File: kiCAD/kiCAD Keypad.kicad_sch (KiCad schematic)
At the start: 71 parts, among them J1 USB_C_Receptacle_USB2.0_16P, J3 2x8 GPIO for SPI, SW1 RESET, SW2 BOOT, SW3 RotaryEncoder_Switch, U1 ESP32-S3-WROOM-2, U2 USBLC6-2SC6, U4 AP2112K-3.3

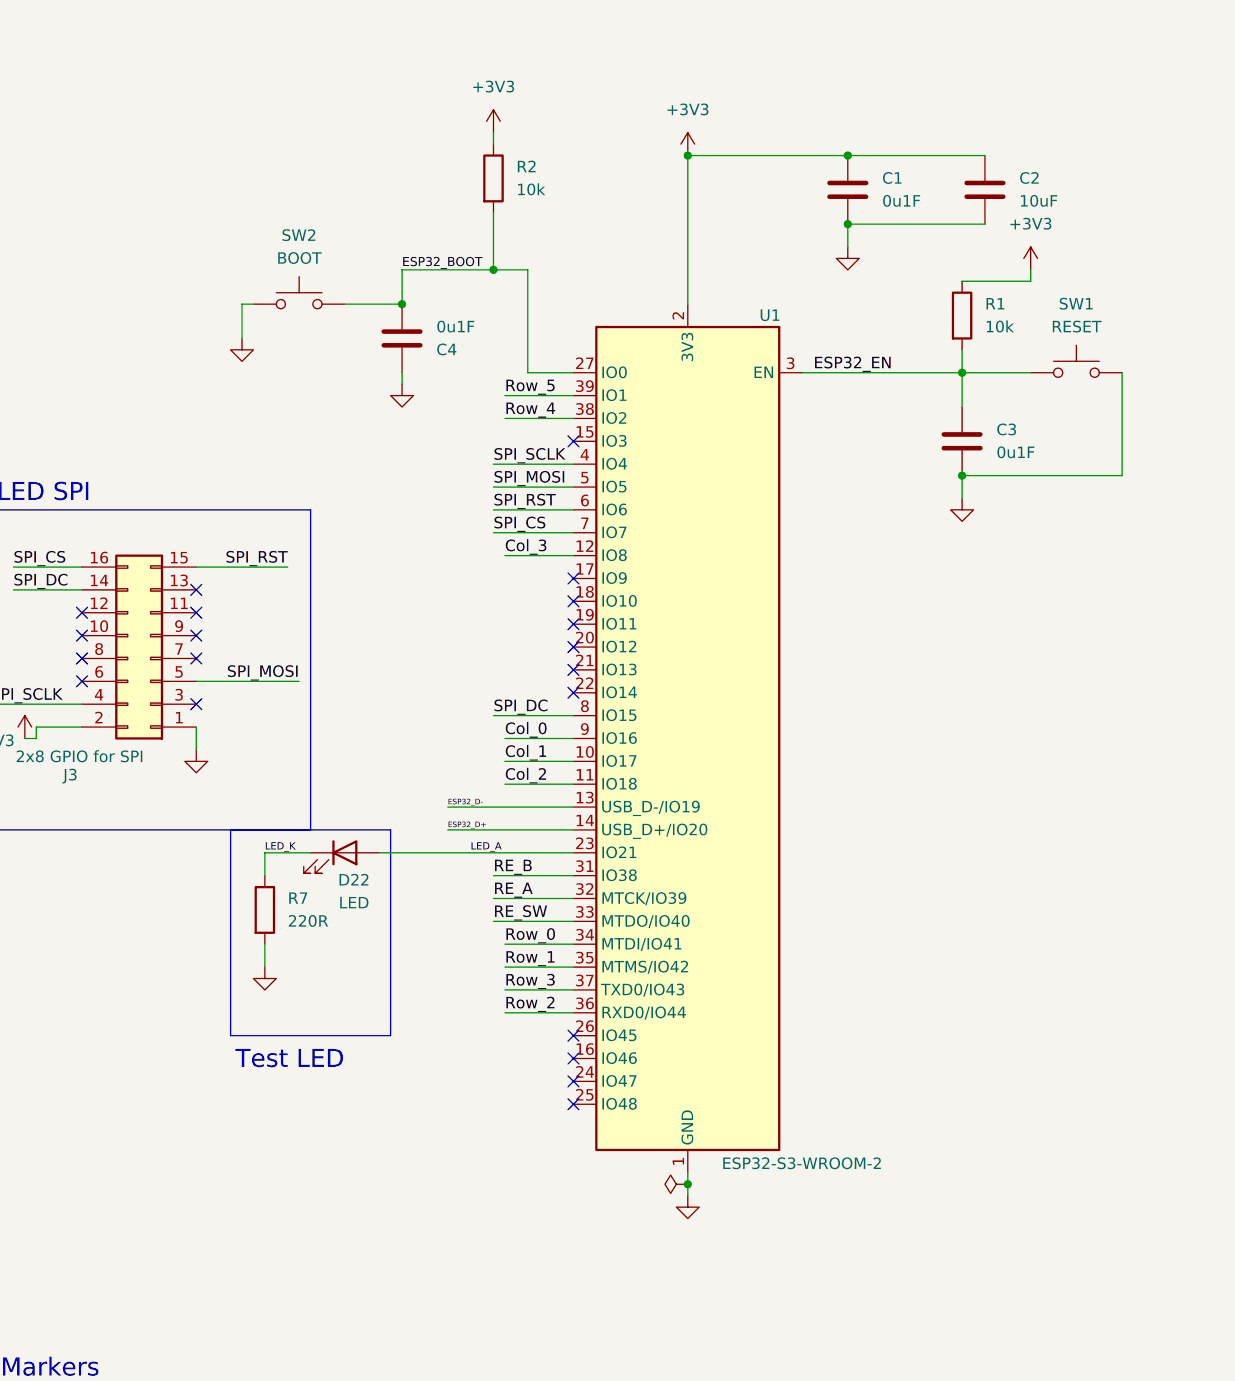
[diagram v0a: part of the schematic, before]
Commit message: Iterating; deciding on switching to devkit
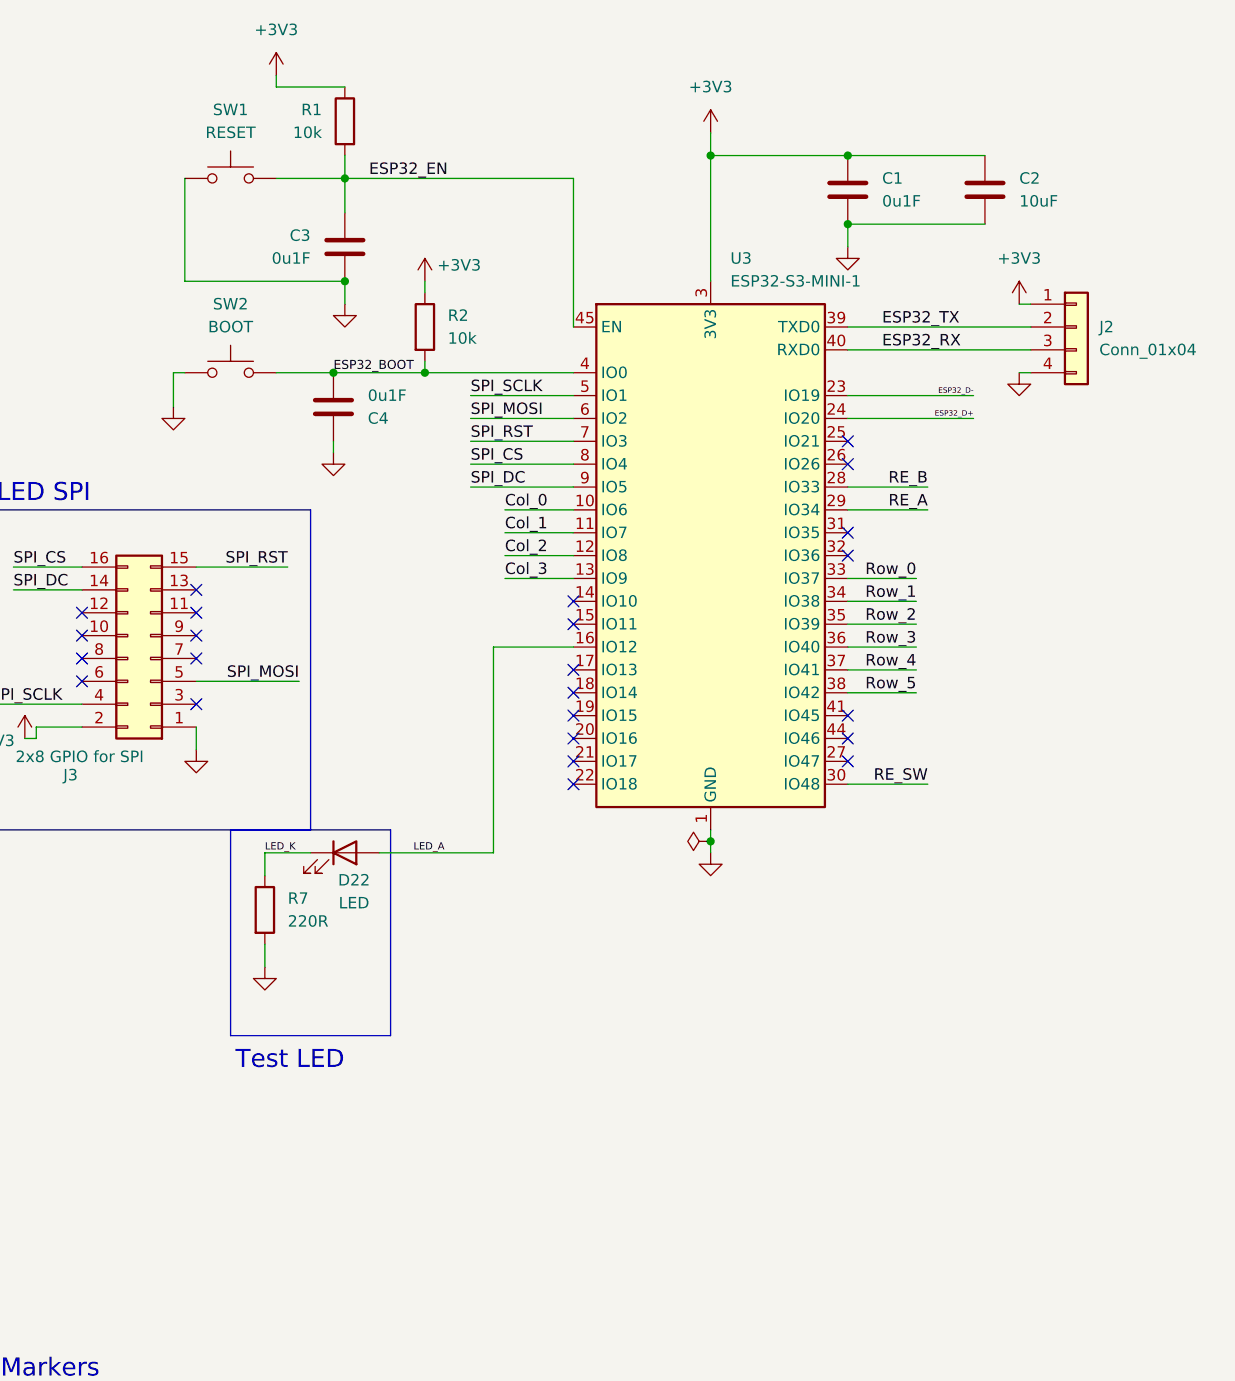
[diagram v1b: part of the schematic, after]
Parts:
- removed U1: ESP32-S3-WROOM-2, RF_Module:ESP32-S3-WROOM-2, symbol RF_Module:ESP32-S3-WROOM-2
- added J2: Conn_01x04, Connector_PinHeader_2.54mm:PinHeader_1x04_P2.54mm_Vertical, symbol Connector_Generic:Conn_01x04
- added U3: ESP32-S3-MINI-1, RF_Module:ESP32-S2-MINI-1, symbol RF_Module:ESP32-S3-MINI-1
- C1, C4: Distributor Link https://www.digikey.com/en/products/detail/nextgen-componen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 -> (none); LCSC (none) -> C1525; Manufacturer Part Number 0402B104K160HI -> (none)
- C2: LCSC (none) -> C408141
- C3: footprint Capacitor_SMD:C_0805_2012Metric -> Capacitor_SMD:C_0402_1005Metric; Distributor Link https://www.digikey.com/en/products/detail/nextgen-componen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 -> (none); LCSC (none) -> C1525; Manufacturer Part Number 0805B105K100CC -> (none)
- C5, C6: LCSC (none) -> C215803; Manufacturer Part Number 0805B105K100CC -> 0805B105K500NT
- D22: LCSC (none) -> C2984137
- J1: LCSC (none) -> C3025063
- J3: LCSC (none) -> C157340
- R1, R2, R5, R6: LCSC (none) -> C98220
- R3, R4: LCSC (none) -> C105580
- R7: LCSC (none) -> C185440
- SW1, SW2: LCSC (none) -> C2799414
- SW3: LCSC (none) -> C143790
- U2: LCSC (none) -> C2827654
- U4: LCSC (none) -> C51118
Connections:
- net +3V3: now also J2.1 (Pin_1), U3.3 (3V3)
- net Col_0: now also U3.10 (IO6)
- net Col_1: now also U3.11 (IO7)
- net Col_2: now also U3.12 (IO8)
- net Col_3: now also U3.13 (IO9)
- net ESP32_BOOT: now also U3.4 (IO0)
- net ESP32_D+: now also U3.24 (IO20)
- net ESP32_D-: now also U3.23 (IO19)
- net ESP32_EN: now also U3.45 (EN)
- net GND: now also J2.4 (Pin_4), U3.1 (GND), U3.2 (GND), U3.42 (GND), U3.43 (GND), U3.46 (GND), U3.47 (GND), U3.48 (GND), U3.49 (GND), U3.50 (GND), U3.51 (GND), U3.52 (GND), U3.53 (GND), U3.54 (GND), U3.55 (GND), U3.56 (GND), U3.57 (GND), U3.58 (GND), U3.59 (GND), U3.60 (GND), U3.61 (GND), U3.62 (GND), U3.63 (GND), U3.64 (GND), U3.65 (GND)
- net LED_A: now also U3.16 (IO12)
- net RE_A: now also U3.29 (IO34)
- net RE_B: now also U3.28 (IO33)
- net RE_SW: now also U3.30 (IO48)
- net Row_0: now also U3.33 (IO37)
- net Row_1: now also U3.34 (IO38)
- net Row_2: now also U3.35 (IO39)
- net Row_3: now also U3.36 (IO40)
- net Row_4: now also U3.37 (IO41)
- net Row_5: now also U3.38 (IO42)
- net SPI_CS: now also U3.8 (IO4)
- net SPI_DC: now also U3.9 (IO5)
- net SPI_MOSI: now also U3.6 (IO2)
- net SPI_RST: now also U3.7 (IO3)
- net SPI_SCLK: now also U3.5 (IO1)
- new net ESP32_RX: J2.3 (Pin_3), U3.40 (RXD0)
- new net ESP32_TX: J2.2 (Pin_2), U3.39 (TXD0)
- no-connect marks 22 -> 26
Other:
- moved on the sheet: C3, C4, R1, R2, SW1, SW2
